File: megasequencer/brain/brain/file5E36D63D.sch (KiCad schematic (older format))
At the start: 23 parts, among them J5 EXT_RATE_CV, J8 EXT_POS_CV, U2 TL074

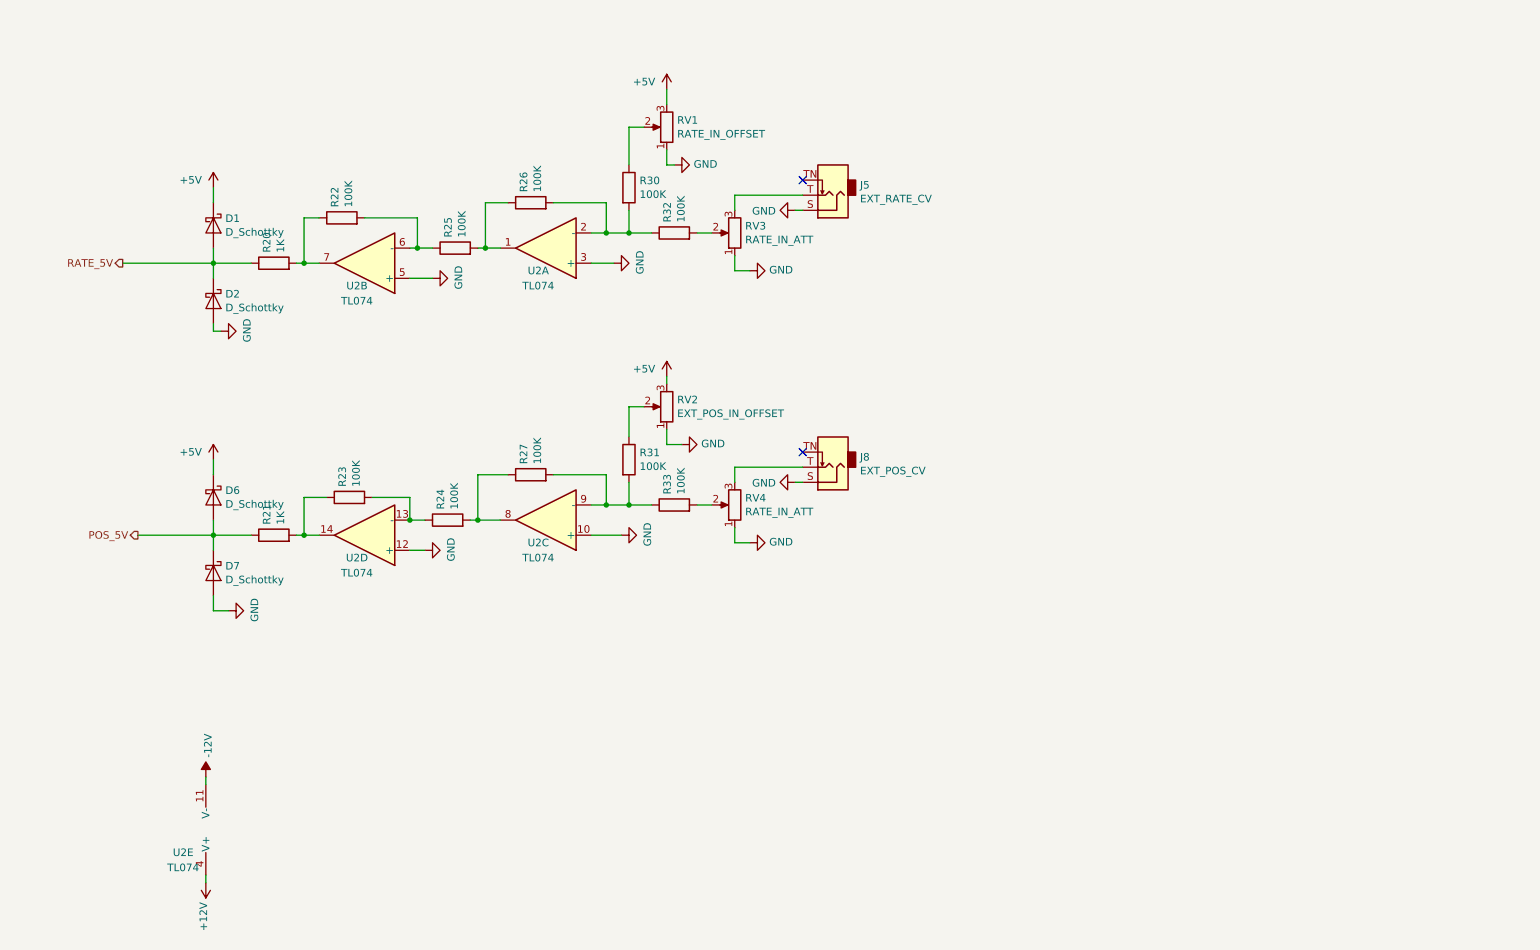
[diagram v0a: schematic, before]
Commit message: Add pwr, more inputs and outputs
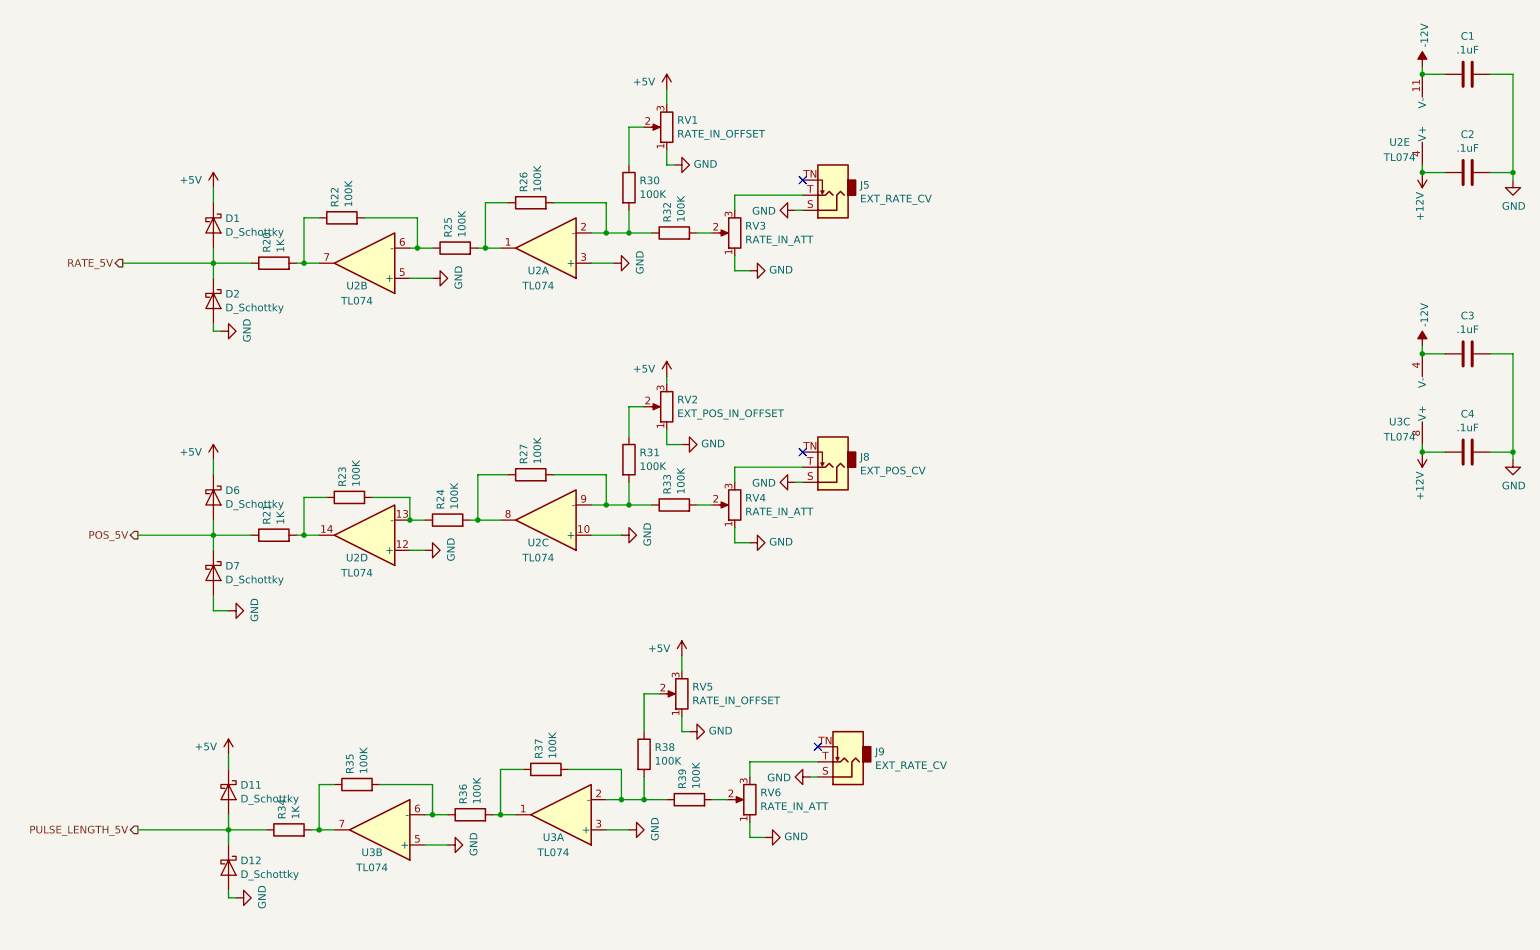
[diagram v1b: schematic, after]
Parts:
- added C1, C2, C3, C4: .1uF, Capacitor_THT:C_Disc_D3.0mm_W1.6mm_P2.50mm, symbol Device:C
- added D11, D12: D_Schottky, Diode_THT:D_DO-34_SOD68_P7.62mm_Horizontal, symbol Device:D_Schottky
- added J9: EXT_RATE_CV, Connector_Audio:Jack_3.5mm_QingPu_WQP-PJ398SM_Vertical_CircularHoles, symbol Connector:AudioJack2_SwitchT
- added R34: 1K, Resistor_THT:R_Axial_DIN0207_L6.3mm_D2.5mm_P7.62mm_Horizontal, symbol Device:R
- added R35, R36, R37, R38, R39: 100K, Resistor_THT:R_Axial_DIN0207_L6.3mm_D2.5mm_P7.62mm_Horizontal, symbol Device:R
- added RV5: RATE_IN_OFFSET, Potentiometer_THT:Potentiometer_Alps_RK09L_Single_Vertical, symbol Device:R_POT
- added RV6: RATE_IN_ATT, Potentiometer_THT:Potentiometer_Alps_RK09L_Single_Vertical, symbol Device:R_POT
- added U3: TL074, Package_DIP:DIP-8_W7.62mm, symbol Amplifier_Operational:TL072
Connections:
- net +12V: now also C2.2, C4.2, U3.8 (V+)
- net +5V: now also D11.1 (K), RV5.3
- net -12V: now also C1.2, C3.2, U3.4 (V-)
- net GND: now also C1.1, C2.1, C3.1, C4.1, D12.2 (A), J9.S, RV5.1, RV6.1, U3.3 (+), U3.5 (+)
- new net: J9.T, RV6.3
- new net: R39.2, RV6.2
- new net: R37.2, R38.2, R39.1, U3.2 (-)
- new net: R38.1, RV5.2
- new net: R36.2, R37.1, U3.1
- new net: R35.2, R36.1, U3.6 (-)
- new net: R34.2, R35.1, U3.7
- new net PULSE_LENGTH_5V: D11.2 (A), D12.1 (K), R34.1
- no-connect marks 2 -> 3
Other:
- moved on the sheet: U2E
